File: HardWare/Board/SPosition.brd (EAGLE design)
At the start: 60 x 110 mm, 72 parts

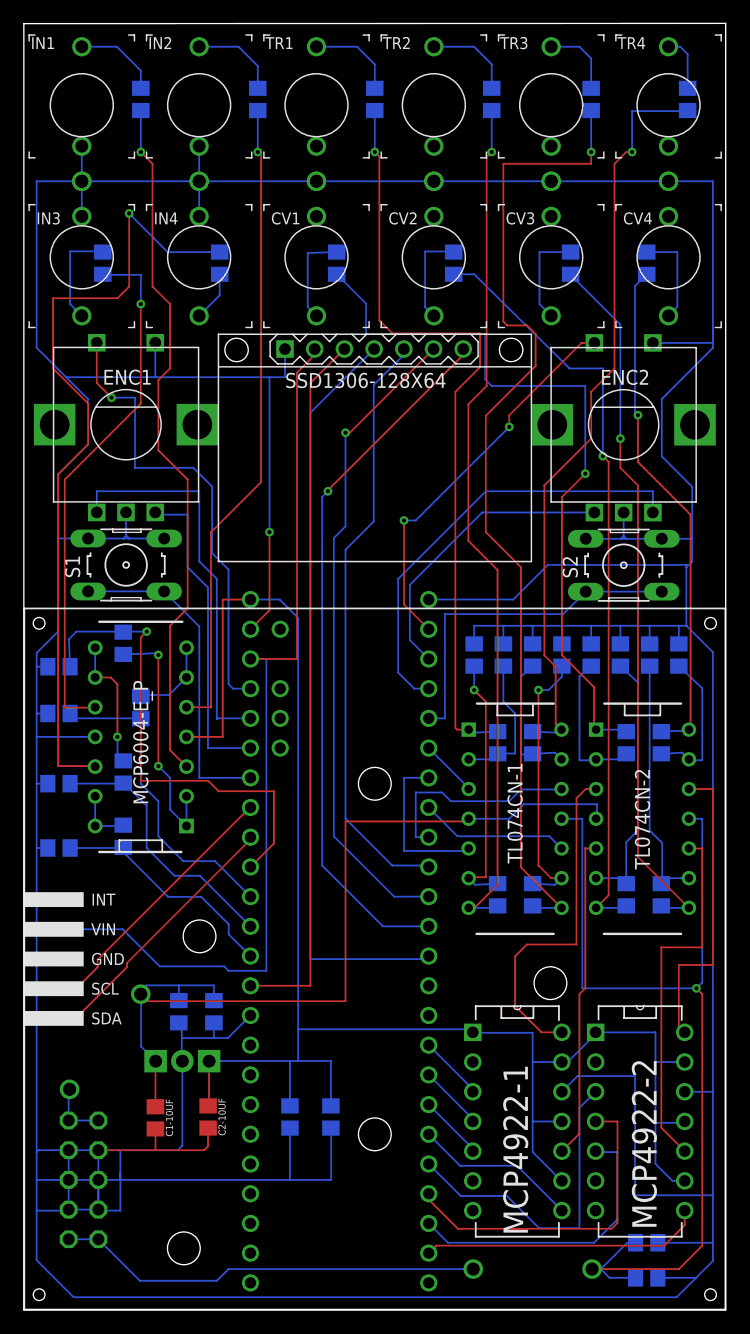
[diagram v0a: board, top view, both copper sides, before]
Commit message: pcb rev5
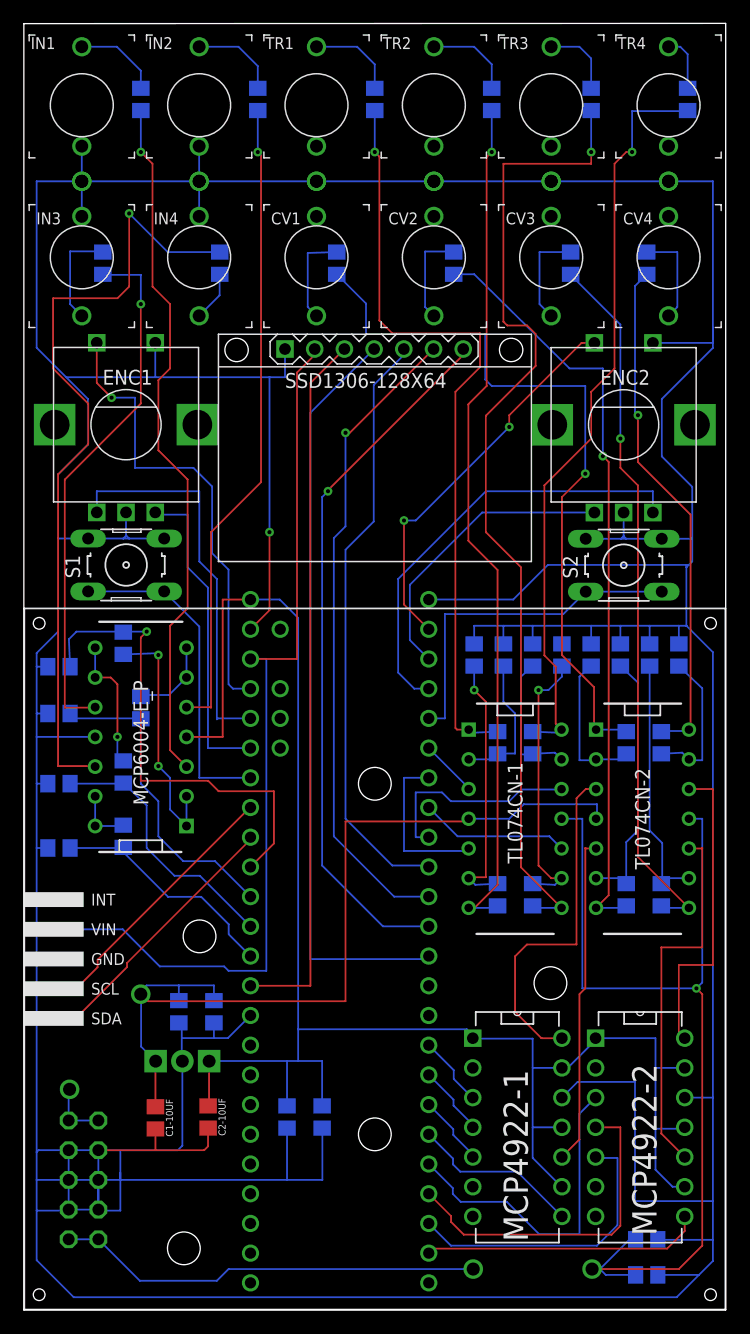
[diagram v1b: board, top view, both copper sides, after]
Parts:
- moved C4-100N 0.75 mm to (25.5, 16.5)
- moved MCP4922-1 0.50 mm to (46.0, 8.00)
- moved MCP4922-2 0.50 mm to (56.5, 8.00)
- moved C3-100N 0.25 mm to (22.5, 16.5)
- moved C7-100N 0.25 mm to (53.2, 3.00)
- moved C8-100N 0.25 mm to (53.2, 6.00)
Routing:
- net DAC2SCK: track 28.4 -> 29.0 mm
- net DAC1CS: track 5.54 -> 6.06 mm
- net DAC1SCK: track 5.54 -> 6.04 mm
- net DAC1MOSI: track 5.54 -> 6.04 mm
- net GND: track 604.1 -> 603.6 mm
- net DAC2CS: track 27.4 -> 27.9 mm
- net DAC1LDAC: track 14.1 -> 14.6 mm
- net CV4: track 31.4 -> 31.9 mm
- net CV3: track 25.9 -> 26.4 mm
- net CV2: track 27.7 -> 28.2 mm
- net CV1: track 29.3 -> 29.8 mm
